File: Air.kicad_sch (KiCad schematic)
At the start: 10 parts

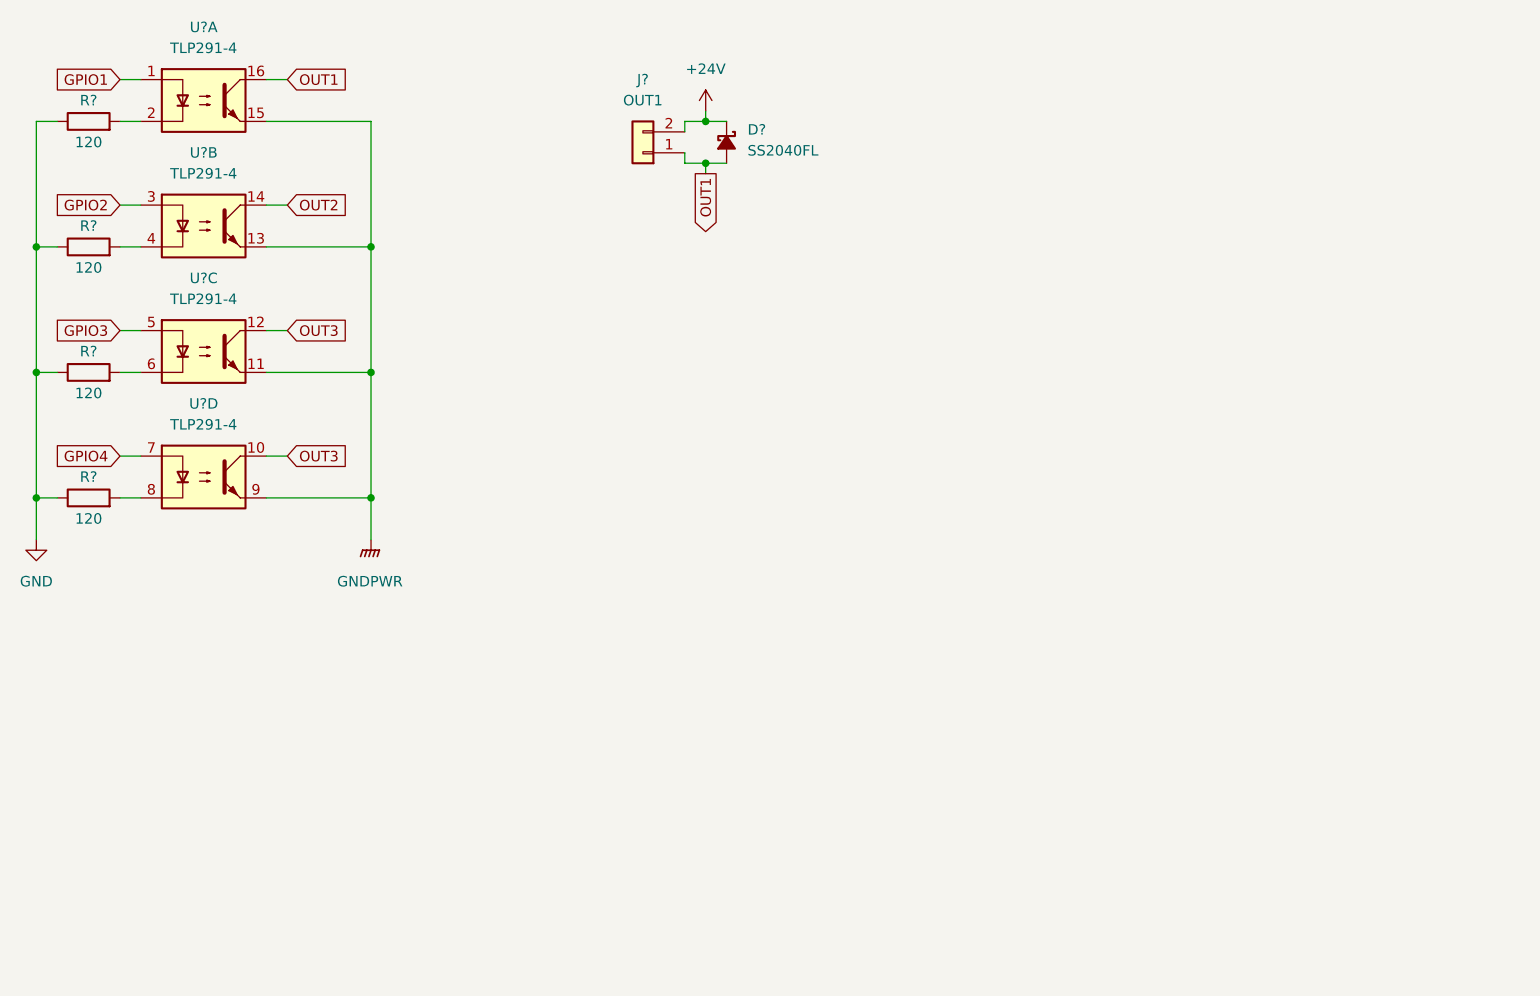
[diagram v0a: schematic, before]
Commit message: chore: Initial commit
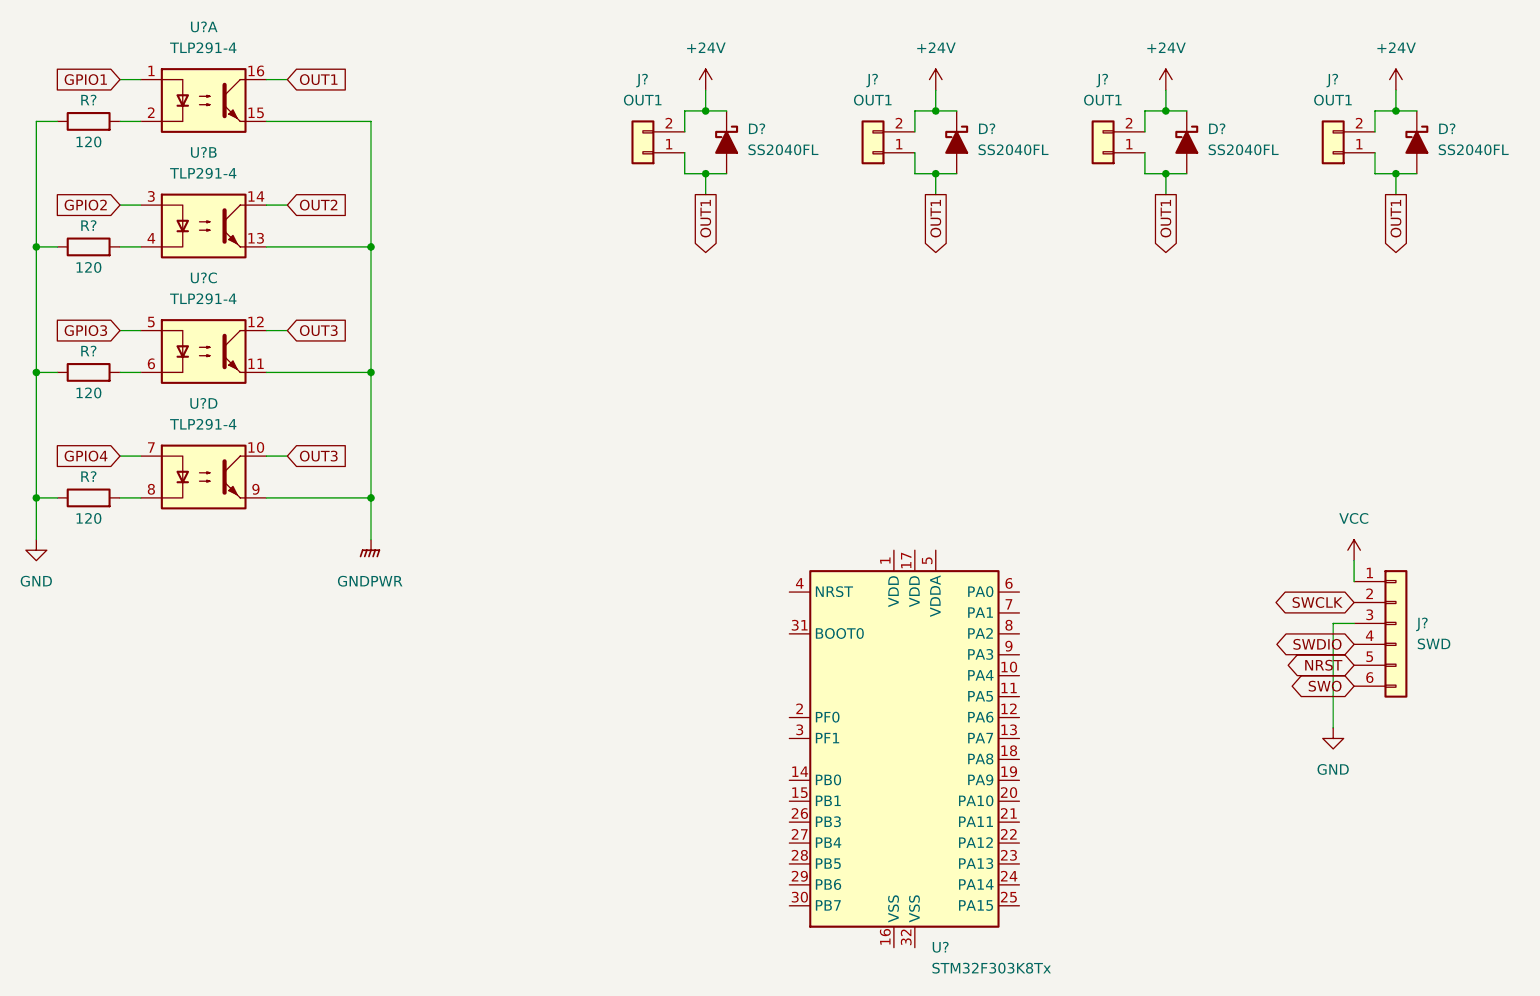
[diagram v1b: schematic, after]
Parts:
- removed D?: SS2040FL, symbol Device:D_Schottky_Small_Filled
- added D? (x4): SS2040FL, symbol Device:D_Schottky_Filled
- added J? (x3): OUT1, symbol Connector_Generic:Conn_01x02
- added J?: SWD, symbol Connector_Generic:Conn_01x06
- added U?: STM32F303K8Tx, Package_QFP:LQFP-32_7x7mm_P0.8mm, symbol MCU_ST_STM32F3:STM32F303K8Tx
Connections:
- net +24V: now also D?.1 (K), D?.1 (K), D?.1 (K), D?.1 (K), J?.2 (Pin_2), J?.2 (Pin_2), J?.2 (Pin_2)
- net GND: now also J?.3 (Pin_3)
- net OUT1: now also D?.2 (A), D?.2 (A), D?.2 (A), D?.2 (A), J?.1 (Pin_1), J?.1 (Pin_1), J?.1 (Pin_1)
- new net NRST: J?.5 (Pin_5)
- new net SWCLK: J?.2 (Pin_2)
- new net SWDIO: J?.4 (Pin_4)
- new net SWO: J?.6 (Pin_6)
- new net VCC: J?.1 (Pin_1)
